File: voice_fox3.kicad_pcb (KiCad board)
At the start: 2 copper layers, 8 parts, among them J2 SJ1-2503A, J3 SJ1-3533NG, Q1 2N3904, U1 DFR0299

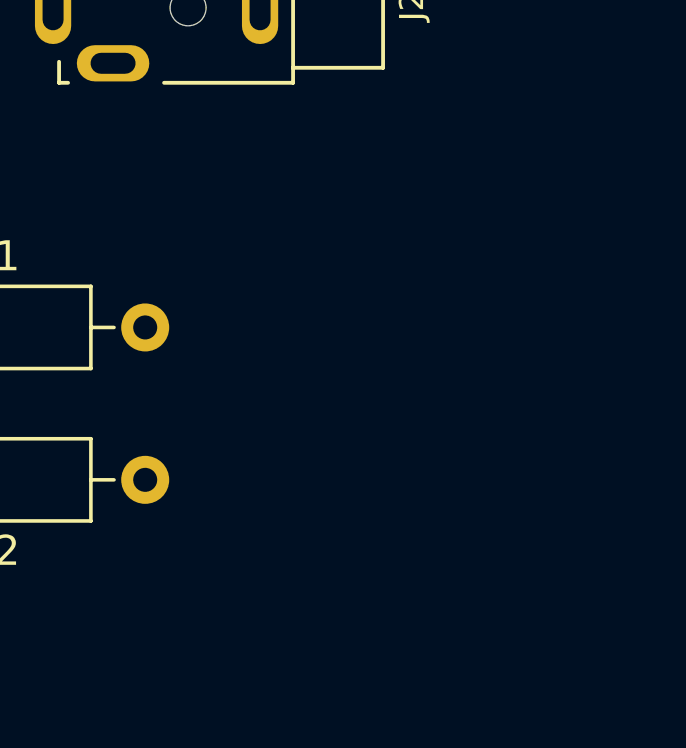
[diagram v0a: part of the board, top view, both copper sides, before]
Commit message: updated pcb from schematic
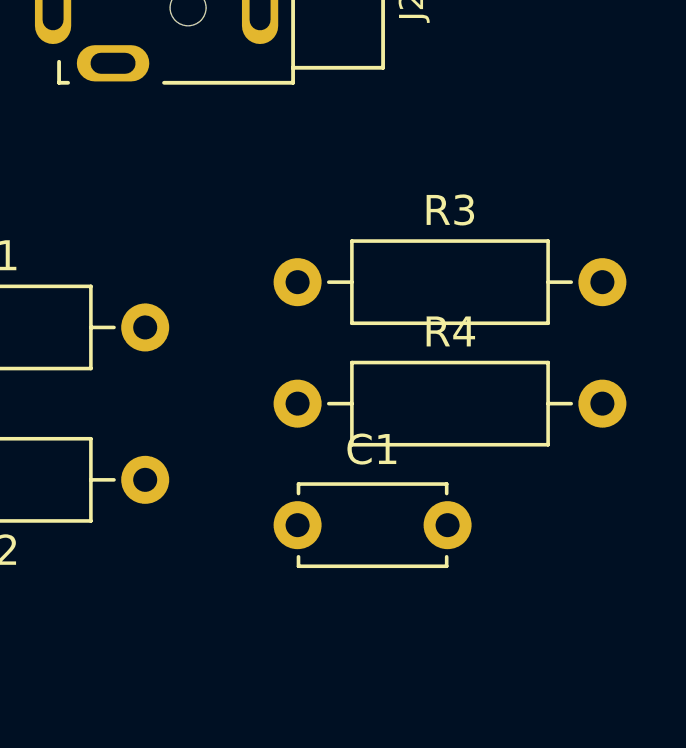
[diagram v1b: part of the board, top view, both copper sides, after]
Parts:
- added C1: 0.1 uf, Capacitor_THT:C_Disc_D4.7mm_W2.5mm_P5.00mm, F.Cu at (162.6, 75.2)
- added R3: 100K, Resistor_THT:R_Axial_DIN0207_L6.3mm_D2.5mm_P10.16mm_Horizontal, F.Cu at (162.6, 67.1)
- added R4: 100K, Resistor_THT:R_Axial_DIN0207_L6.3mm_D2.5mm_P10.16mm_Horizontal, F.Cu at (162.6, 71.1)
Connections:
- A2 pad J1_1: unconnected-(A2A-A0-PadJ1_1) -> Net-(A2A-A0)
- A2 pad J1_11: unconnected-(A2A-3V3-PadJ1_11) -> +3.3V
- A2 pad J2_15: Net-(U1-VCC) -> +3.3V
- A2 pad J2_6: Net-(U1-VCC) -> +3.3V
- J2 pad 3: unconnected-(J2-Pad3) -> Net-(C1-Pad2)
- U1 pad 1: Net-(U1-VCC) -> +3.3V

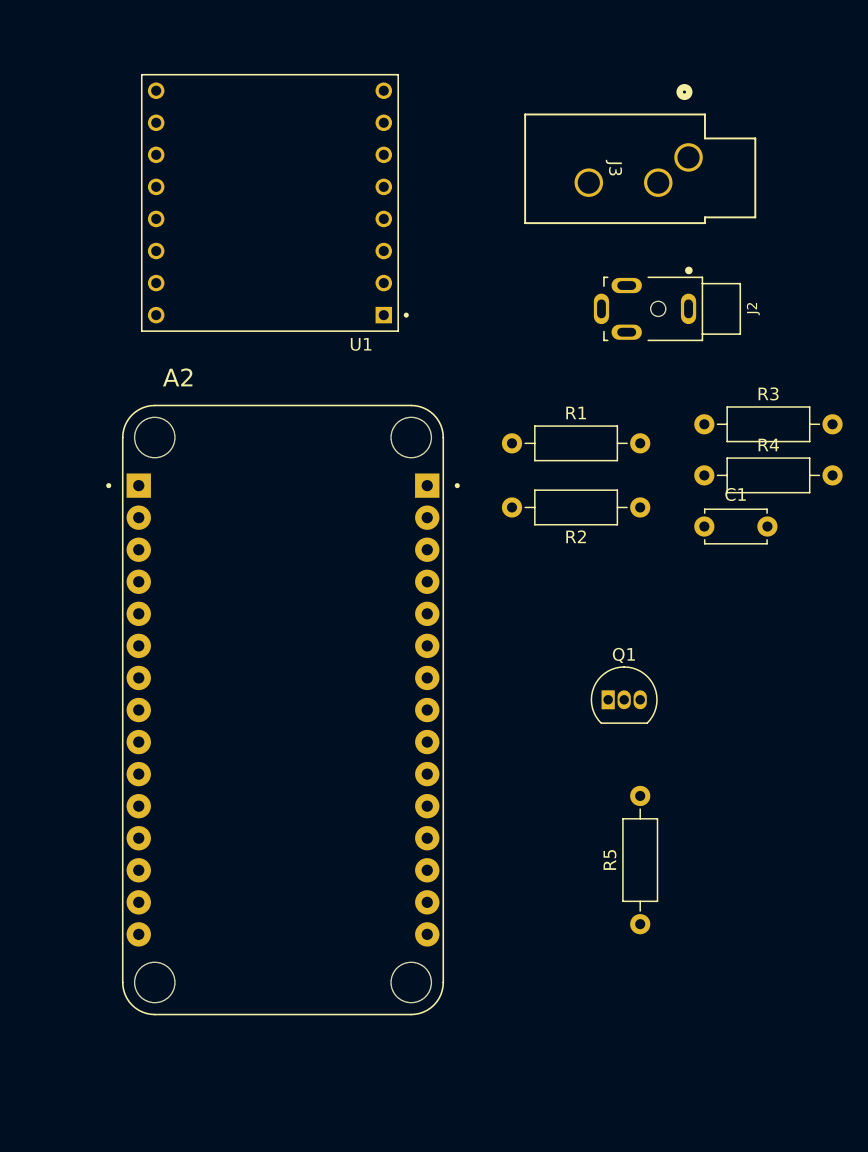
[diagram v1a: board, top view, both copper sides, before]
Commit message: initial placement
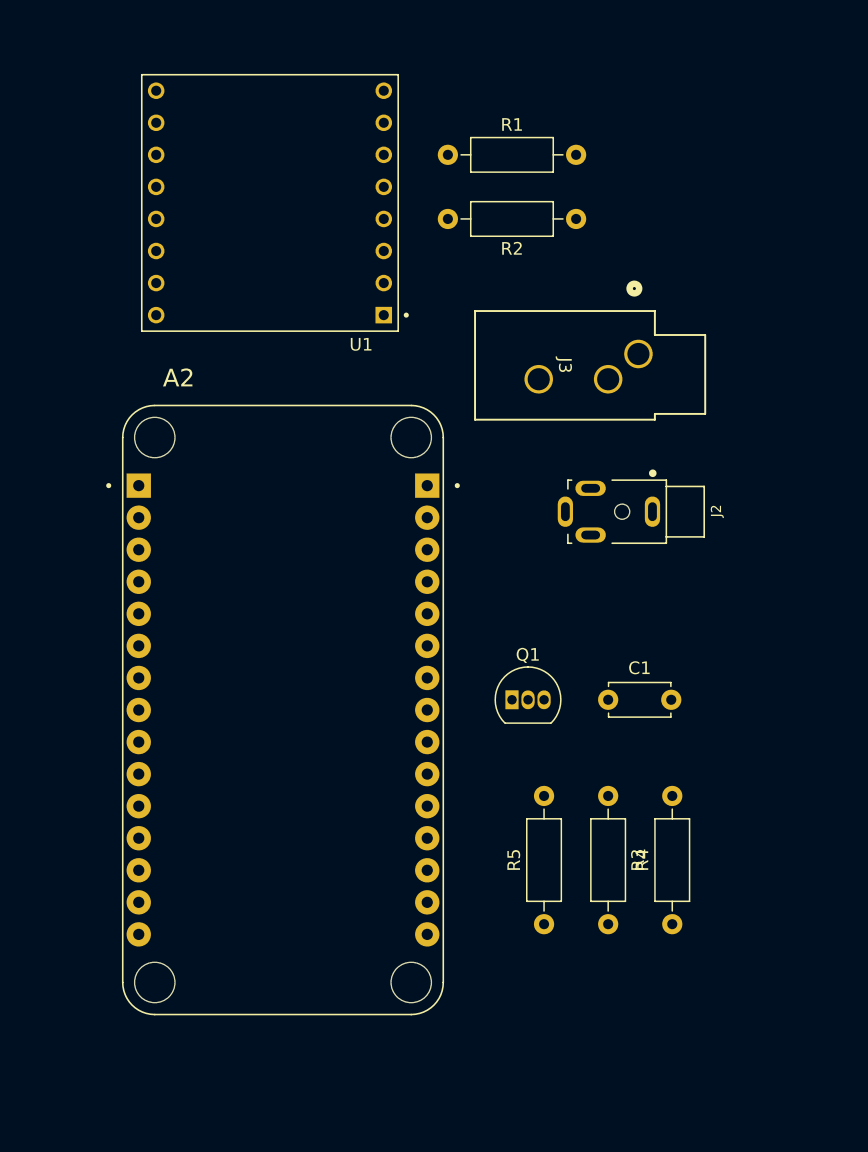
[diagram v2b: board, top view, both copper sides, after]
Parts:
- moved R4 35.7 mm to (160.0, 106.7), turned to 90 degrees
- moved R3 30.4 mm to (154.9, 96.5), turned to -90 degrees
- moved R1 23.4 mm to (142.2, 45.7)
- moved R2 23.4 mm to (152.4, 50.8)
- moved J2 16.3 mm to (158.5, 74.0)
- moved J3 16.1 mm to (157.3, 61.5)
- moved C1 15.7 mm to (154.9, 88.9)
- moved Q1 7.62 mm to (147.3, 88.9)
- moved R5 7.62 mm to (149.9, 106.7)
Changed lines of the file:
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@@
   (net 42 "Net-(Q1-C)")
   (footprint "bills_library:CUI_SJ1-2503A" (layer "F.Cu")
-    (at 161.309206 57.924899 -90)
+    (at 158.450792 73.9951 -90)
     (property "MANUFACTURER" "CUI INC")
     (property "REV" "B")
@@
   )
   (footprint "Resistor_THT:R_Axial_DIN0207_L6.3mm_D2.5mm_P10.16mm_Horizontal" (layer "F.Cu")
-    (at 162.56 71.12)
+    (at 160.02 106.68 90)
     (descr "Resistor, Axial_DIN0207 series, Axial, Horizontal, pin pitch=10.16mm, 0.25W = 1/4W, length*diameter=6.3*2.5mm^2, http://cdn-reichelt.de/documents/datenblatt/B400/1_4W%23YAG.pdf")
     (tags "Resistor Axial_DIN0207 series Axial Horizontal pin pitch 10.16mm 0.25W = 1/4W length 6.3mm diameter 2.5mm")
@@
     (property "ki_keywords" "R res resistor")
     (attr through_hole)
-    (fp_text reference "R4" (at 5.08 -2.37) (layer "F.SilkS")
-        (effects (font (size 1 1) (thickness 0.15)))
-    )
-    (fp_text value "100K" (at 5.08 2.37) (layer "F.Fab")
-        (effects (font (size 1 1) (thickness 0.15)))
-    )
-    (fp_text user "${REFERENCE}" (at 5.08 0) (layer "F.Fab")
+    (fp_text reference "R4" (at 5.08 -2.37 90) (layer "F.SilkS")
+        (effects (font (size 1 1) (thickness 0.15)))
+    )
+    (fp_text value "100K" (at 5.08 2.37 90) (layer "F.Fab")
+        (effects (font (size 1 1) (thickness 0.15)))
+    )
+    (fp_text user "${REFERENCE}" (at 5.08 0 90) (layer "F.Fab")
         (effects (font (size 1 1) (thickness 0.15)))
     )
@@
     (fp_line (start 10.16 0) (end 8.23 0)
       (stroke (width 0.1) (type solid)) (layer "F.Fab"))
-    (pad "1" thru_hole circle (at 0 0) (size 1.6 1.6) (drill 0.8) (layers "*.Cu" "*.Mask")
+    (pad "1" thru_hole circle (at 0 0 90) (size 1.6 1.6) (drill 0.8) (layers "*.Cu" "*.Mask")
       (net 11 "+3.3V") (pintype "passive"))
-    (pad "2" thru_hole oval (at 10.16 0) (size 1.6 1.6) (drill 0.8) (layers "*.Cu" "*.Mask")
+    (pad "2" thru_hole oval (at 10.16 0 90) (size 1.6 1.6) (drill 0.8) (layers "*.Cu" "*.Mask")
       (net 1 "Net-(A2A-A0)") (pintype "passive"))
     (model "${KICAD6_3DMODEL_DIR}/Resistor_THT.3dshapes/R_Axial_DIN0207_L6.3mm_D2.5mm_P10.16mm_Horizontal.wrl"
@@
   )
   (footprint "bills_library:SJ1-3533NG_CUD" (layer "F.Cu")
-    (at 161.309206 45.924899 -90)
+    (at 157.339998 61.499999 -90)
     (tags "SJ1-3533NG ")
     (property "Sheetfile" "voice_fox3.kicad_sch")
@@
   )
   (footprint "Resistor_THT:R_Axial_DIN0207_L6.3mm_D2.5mm_P10.16mm_Horizontal" (layer "F.Cu")
-    (at 157.48 106.68 90)
+    (at 149.86 106.68 90)
     (descr "Resistor, Axial_DIN0207 series, Axial, Horizontal, pin pitch=10.16mm, 0.25W = 1/4W, length*diameter=6.3*2.5mm^2, http://cdn-reichelt.de/documents/datenblatt/B400/1_4W%23YAG.pdf")
     (tags "Resistor Axial_DIN0207 series Axial Horizontal pin pitch 10.16mm 0.25W = 1/4W length 6.3mm diameter 2.5mm")
@@
   )
   (footprint "Package_TO_SOT_THT:TO-92_Inline" (layer "F.Cu")
-    (at 154.94 88.9)
+    (at 147.32 88.9)
     (descr "TO-92 leads in-line, narrow, oval pads, drill 0.75mm (see NXP sot054_po.pdf)")
     (tags "to-92 sc-43 sc-43a sot54 PA33 transistor")
@@
   )
   (footprint "Capacitor_THT:C_Disc_D4.7mm_W2.5mm_P5.00mm" (layer "F.Cu")
-    (at 162.56 75.17)
+    (at 154.94 88.9)
     (descr "C, Disc series, Radial, pin pitch=5.00mm, , diameter*width=4.7*2.5mm^2, Capacitor, http://www.vishay.com/docs/45233/krseries.pdf")
     (tags "C Disc series Radial pin pitch 5.00mm  diameter 4.7mm width 2.5mm Capacitor")
@@
   )
   (footprint "Resistor_THT:R_Axial_DIN0207_L6.3mm_D2.5mm_P10.16mm_Horizontal" (layer "F.Cu")
-    (at 147.32 68.58)
+    (at 142.24 45.72)
     (descr "Resistor, Axial_DIN0207 series, Axial, Horizontal, pin pitch=10.16mm, 0.25W = 1/4W, length*diameter=6.3*2.5mm^2, http://cdn-reichelt.de/documents/datenblatt/B400/1_4W%23YAG.pdf")
     (tags "Resistor Axial_DIN0207 series Axial Horizontal pin pitch 10.16mm 0.25W = 1/4W length 6.3mm diameter 2.5mm")
@@
   )
   (footprint "Resistor_THT:R_Axial_DIN0207_L6.3mm_D2.5mm_P10.16mm_Horizontal" (layer "F.Cu")
-    (at 157.48 73.66 180)
+    (at 152.4 50.8 180)
     (descr "Resistor, Axial_DIN0207 series, Axial, Horizontal, pin pitch=10.16mm, 0.25W = 1/4W, length*diameter=6.3*2.5mm^2, http://cdn-reichelt.de/documents/datenblatt/B400/1_4W%23YAG.pdf")
     (tags "Resistor Axial_DIN0207 series Axial Horizontal pin pitch 10.16mm 0.25W = 1/4W length 6.3mm diameter 2.5mm")
@@
   )
   (footprint "Resistor_THT:R_Axial_DIN0207_L6.3mm_D2.5mm_P10.16mm_Horizontal" (layer "F.Cu")
-    (at 162.56 67.07)
+    (at 154.94 96.52 -90)
     (descr "Resistor, Axial_DIN0207 series, Axial, Horizontal, pin pitch=10.16mm, 0.25W = 1/4W, length*diameter=6.3*2.5mm^2, http://cdn-reichelt.de/documents/datenblatt/B400/1_4W%23YAG.pdf")
     (tags "Resistor Axial_DIN0207 series Axial Horizontal pin pitch 10.16mm 0.25W = 1/4W length 6.3mm diameter 2.5mm")
@@
     (property "ki_keywords" "R res resistor")
     (attr through_hole)
-    (fp_text reference "R3" (at 5.08 -2.37) (layer "F.SilkS")
-        (effects (font (size 1 1) (thickness 0.15)))
-    )
-    (fp_text value "100K" (at 5.08 2.37) (layer "F.Fab")
-        (effects (font (size 1 1) (thickness 0.15)))
-    )
-    (fp_text user "${REFERENCE}" (at 5.08 0) (layer "F.Fab")
+    (fp_text reference "R3" (at 5.08 -2.37 90) (layer "F.SilkS")
+        (effects (font (size 1 1) (thickness 0.15)))
+    )
+    (fp_text value "100K" (at 5.08 2.37 90) (layer "F.Fab")
+        (effects (font (size 1 1) (thickness 0.15)))
+    )
+    (fp_text user "${REFERENCE}" (at 5.08 0 90) (layer "F.Fab")
         (effects (font (size 1 1) (thickness 0.15)))
     )
@@
     (fp_line (start 10.16 0) (end 8.23 0)
       (stroke (width 0.1) (type solid)) (layer "F.Fab"))
-    (pad "1" thru_hole circle (at 0 0) (size 1.6 1.6) (drill 0.8) (layers "*.Cu" "*.Mask")
+    (pad "1" thru_hole circle (at 0 0 270) (size 1.6 1.6) (drill 0.8) (layers "*.Cu" "*.Mask")
       (net 1 "Net-(A2A-A0)") (pintype "passive"))
-    (pad "2" thru_hole oval (at 10.16 0) (size 1.6 1.6) (drill 0.8) (layers "*.Cu" "*.Mask")
+    (pad "2" thru_hole oval (at 10.16 0 270) (size 1.6 1.6) (drill 0.8) (layers "*.Cu" "*.Mask")
       (net 10 "GND") (pintype "passive"))
     (model "${KICAD6_3DMODEL_DIR}/Resistor_THT.3dshapes/R_Axial_DIN0207_L6.3mm_D2.5mm_P10.16mm_Horizontal.wrl"

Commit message: many changes
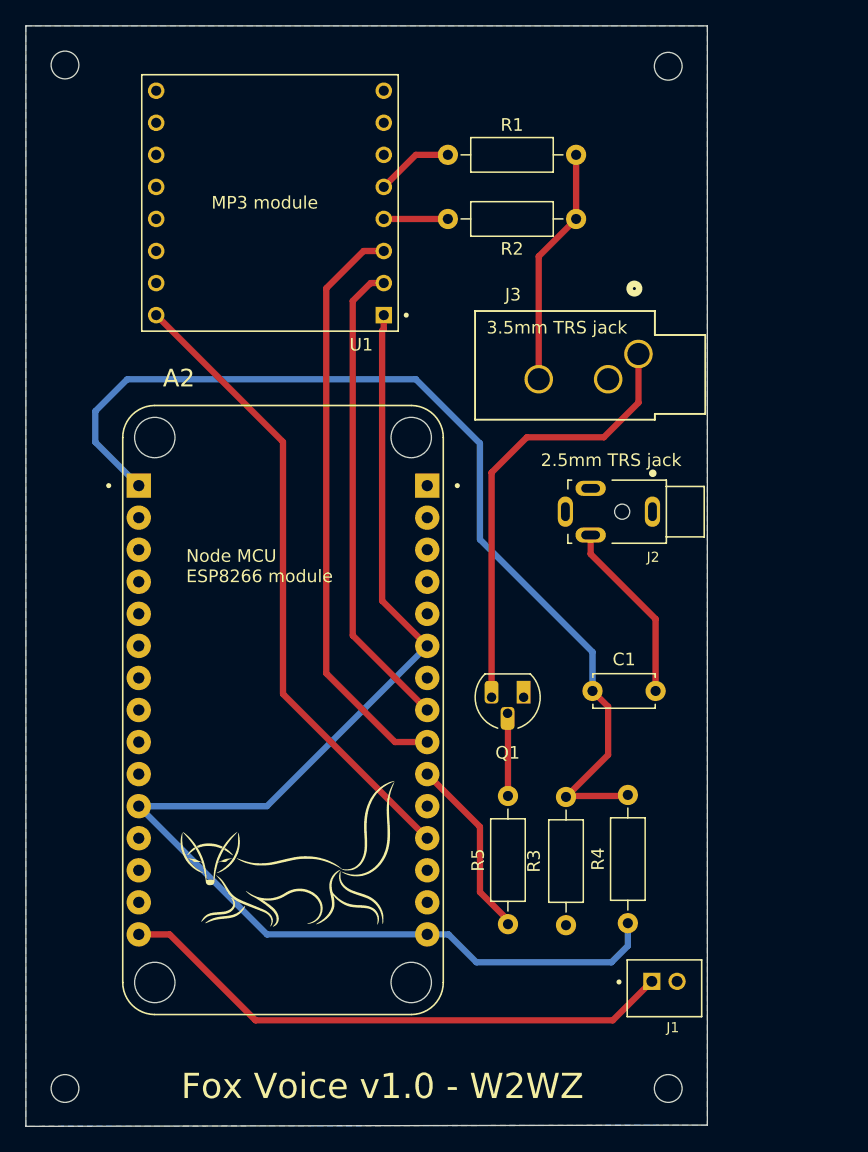
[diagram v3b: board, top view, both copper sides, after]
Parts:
- added G***: LOGO, LOGO, F.Cu at (129.5, 101.1)
- added H0: MountingHole_2.2mm_M2, MountingHole:MountingHole_2.2mm_M2, F.Cu at (111.9, 38.6)
- added H1: MountingHole_2.2mm_M2, MountingHole:MountingHole_2.2mm_M2, F.Cu at (159.7, 38.7)
- added H2: MountingHole_2.2mm_M2, MountingHole:MountingHole_2.2mm_M2, F.Cu at (111.9, 119.7)
- added H3: MountingHole_2.2mm_M2, MountingHole:MountingHole_2.2mm_M2, F.Cu at (159.7, 119.7)
- added J1: 2 pin 2mm JST, bills_library:JST_B2B-PH-K-S(LF)(SN), F.Cu at (159.4, 111.8)
- Q1: footprint Package_TO_SOT_THT:TO-92_Inline -> Package_TO_SOT_THT:TO-92_HandSolder
- moved R4 3.52 mm to (156.5, 106.6)
- moved R3 3.34 mm to (151.6, 96.6)
- moved R5 2.86 mm to (147.0, 106.7)
- moved C1 1.42 mm to (153.7, 88.2)
- moved Q1 0.94 mm to (148.2, 88.7), turned to 180 degrees
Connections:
- A2 pad J1_15: unconnected-(A2A-VIN-PadJ1_15) -> Net-(A2A-VIN)
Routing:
- net +3.3V: track 0.00 -> 102.1 mm
- net Net-(A2A-A0): track 0.00 -> 79.5 mm
- net Net-(A2B-D9): track 0.00 -> 50.3 mm
- net Net-(A2B-D6): track 0.00 -> 46.5 mm
- net Net-(A2A-VIN): track 0.00 -> 44.8 mm
- net Net-(A2B-D5): track 0.00 -> 37.9 mm
- net Net-(Q1-C): track 0.00 -> 35.6 mm
- net Net-(J3-Pad3): track 0.00 -> 19.0 mm
- net Net-(A2B-D7): track 0.00 -> 14.5 mm
- net Net-(C1-Pad2): track 0.00 -> 14.5 mm
- net Net-(Q1-B): track 0.00 -> 6.56 mm
- net Net-(U1-DAC_L): track 0.00 -> 6.13 mm
- net Net-(U1-DAC_R): track 0.00 -> 5.08 mm
- added copper zone on B.Cu, net GND
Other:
- board outline added: 54 x 87.2 mm
- board text added: "2.5mm TRS jack"
- board text added: "3.5mm TRS jack"
- board text added: "Fox Voice v1.0 - W2WZ"
- board text added: "MP3 module"
- board text added: "Node MCU ESP8266 module"
